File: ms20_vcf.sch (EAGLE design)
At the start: 27 parts, among them IC1 LM13700N, IC2 TL082P, IC3 TL082P, Q1 BC559C, Q2 BC559C

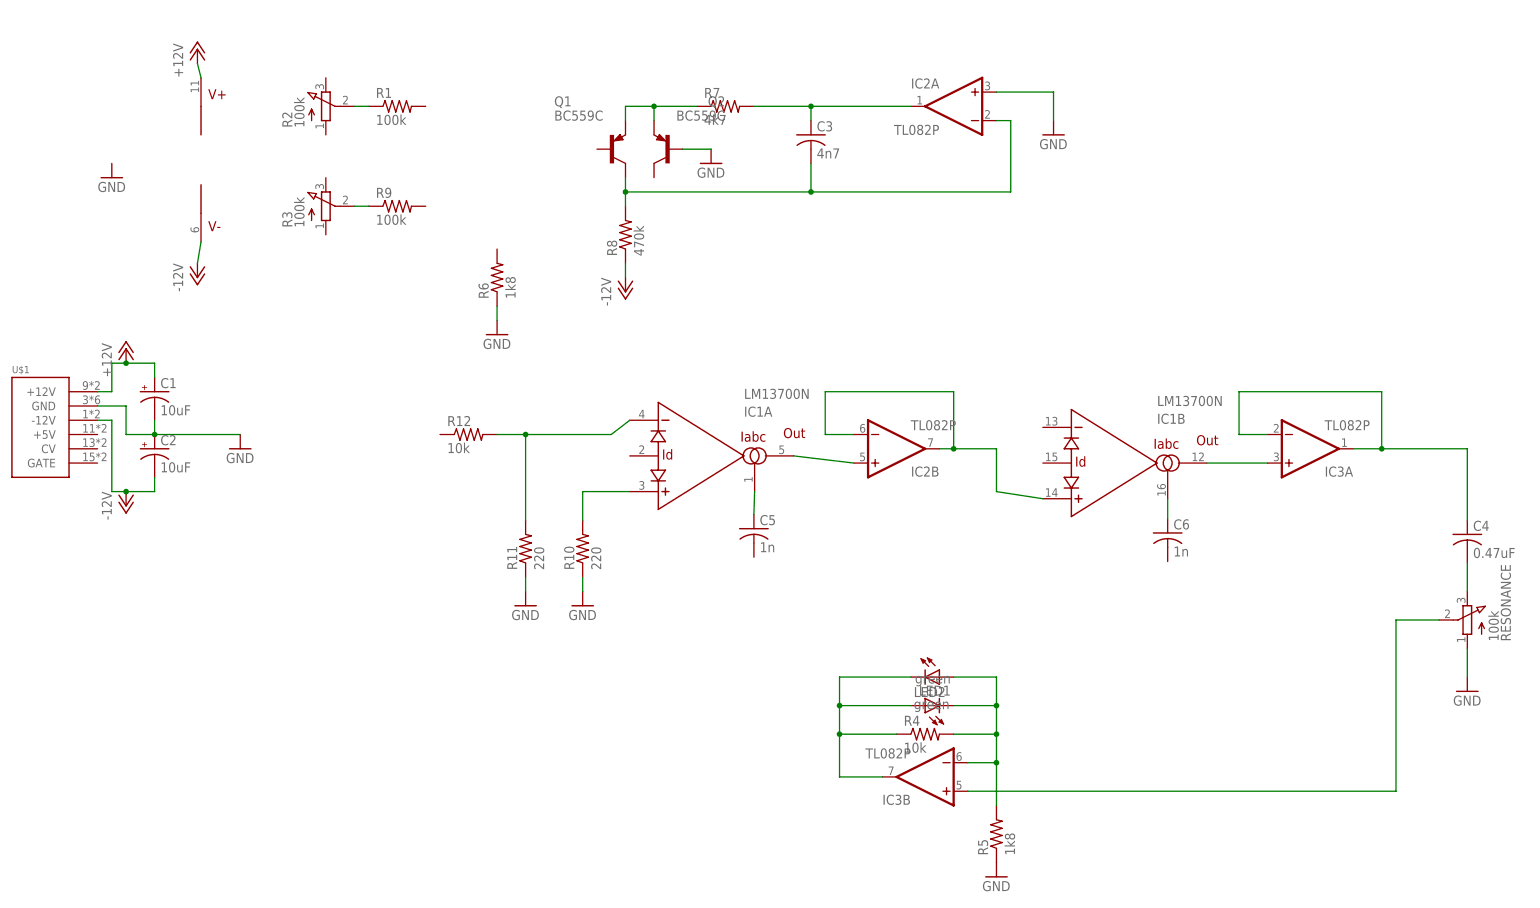
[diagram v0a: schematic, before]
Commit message: all but jacks complete
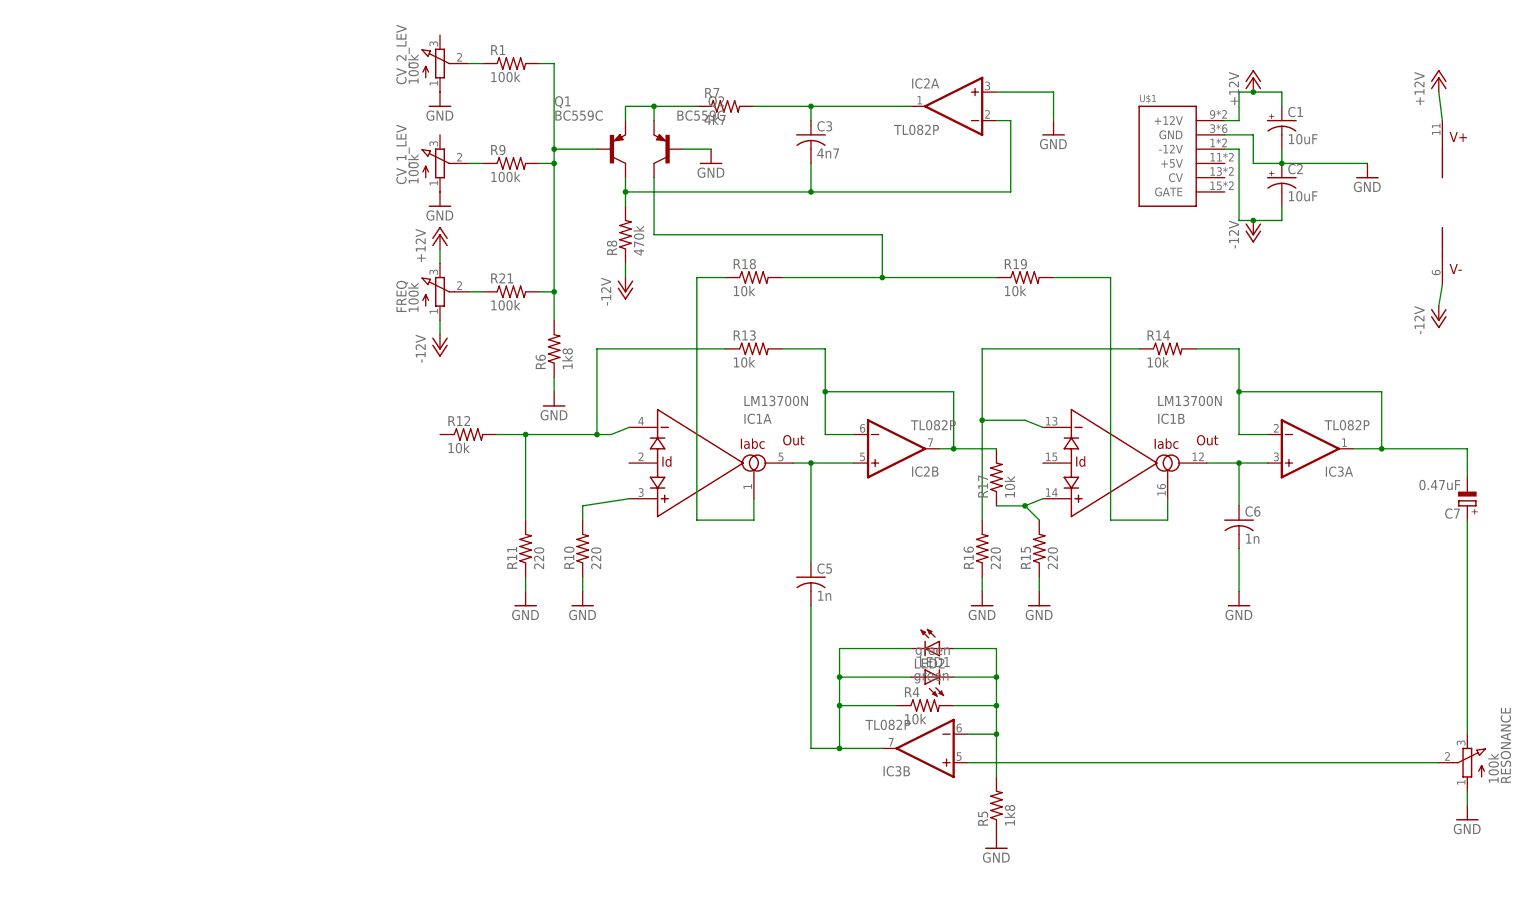
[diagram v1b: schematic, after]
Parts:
- removed C4: 0.47uF, rcl:C-US050-024X044
- removed R2, R3: 100k, pot:3RP/1610N
- added C7: 0.47uF, rcl:CPOL-EUB45181A
- added CV_1_LEV, CV_2_LEV, FREQ: 100k, pot:3RP/1610N
- added R13, R14, R17, R18, R19: 10k, rcl:R-US_0207/10
- added R15, R16: 220, rcl:R-US_0207/10
- added R21: 100k, rcl:R-US_0207/10
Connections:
- new net N$18: IC1B.-IN, R14.1, R16.2
- new net N$19: IC2B.-IN, IC2B.OUT, R13.2, R17.2
- new net N$20: IC1B.+IN, R15.2, R17.1
- new net N$21: Q1.B, R1.2, R21.2, R6.2, R9.2
- new net N$22: FREQ.S, R21.1
- net +12V: now also FREQ.E
- net -12V: now also FREQ.A
- net GND: now also C6.2, CV_1_LEV.A, CV_2_LEV.A, R15.1, R16.1
- net N$10: now also C6.1
- net N$11: now also C7.-, R14.2; no longer C4.1
- net N$12: now also C7.+; no longer C4.2
- net N$13: now also R18.1; no longer C5.1
- net N$14: now also R13.1
- net N$16: now also Q2.C, R18.2, R19.1; no longer IC1B.+IN, IC2B.-IN, IC2B.OUT
- net N$17: now also R19.2; no longer C6.1
- net N$2: now also C5.2
- net N$7: now also CV_2_LEV.S; no longer R2.S
- net N$8: now also CV_1_LEV.S; no longer R3.S
- net N$9: now also C5.1
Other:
- moved on the sheet: C1, C2, C5, C6, IC1A, IC3B, LED1, LED2, R1, R4, R5, R6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
